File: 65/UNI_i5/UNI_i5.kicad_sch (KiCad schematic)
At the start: 191 parts, among them J2 Conn_01x04, J3 Conn_01x05, SW1 MX_SW_solder, SW10 MX_SW_solder, SW11 MX_SW_solder, SW12 MX_SW_solder, SW13 MX_SW_solder, SW14 MX_SW_solder, SW15 MX_SW_solder, SW16 MX_SW_solder, SW17 MX_SW_solder, SW18 MX_SW_solder, SW19 MX_SW_solder, SW2 MX_SW_solder, SW20 MX_SW_solder, SW21 MX_SW_solder, SW22 MX_SW_solder, SW23 MX_SW_solder, SW24 MX_SW_solder, SW25 MX_SW_solder, SW26 MX_SW_solder, SW27 MX_SW_solder, SW28 MX_SW_solder, SW29 MX_SW_solder, SW3 MX_SW_solder, SW30 MX_SW_solder, SW31 MX_SW_solder, SW32 RotaryEncoder_Switch, SW33 MX_SW_solder, SW34 MX_SW_solder, SW35 MX_SW_solder, SW36 MX_SW_solder, SW37 MX_SW_solder, SW38 MX_SW_solder, SW39 MX_SW_solder, SW4 MX_SW_solder, SW40 MX_SW_solder, SW41 MX_SW_solder, SW42 MX_SW_solder, SW43 MX_SW_solder, SW44 MX_SW_solder, SW45 MX_SW_solder, SW46 MX_SW_solder, SW47 MX_SW_solder, SW48 RotaryEncoder_Switch, SW49 MX_SW_solder, SW5 MX_SW_solder, SW50 MX_SW_solder, SW51 MX_SW_solder, SW52 MX_SW_solder, SW53 MX_SW_solder, SW54 MX_SW_solder, SW55 MX_SW_solder, SW56 MX_SW_solder, SW57 MX_SW_solder, SW58 MX_SW_solder, SW59 MX_SW_solder, SW6 MX_SW_solder, SW60 MX_SW_solder, SW61 MX_SW_solder, SW62 MX_SW_solder, SW63 MX_SW_solder, SW64 MX_SW_solder, SW65 MX_SW_solder, SW66 MX_SW_solder, SW67 MX_SW_solder, SW68 MX_SW_solder, SW69 MX_SW_solder, SW7 MX_SW_solder, SW70 MX_SW_solder, SW71 MX_SW_solder, SW72 MX_SW_solder, SW73 MX_SW_solder, SW74 MX_SW_solder, SW75 MX_SW_solder, SW76 SW_RESET, SW77 SW_BOOTSEL, SW8 MX_SW_solder, SW9 MX_SW_solder, U1 RP2040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

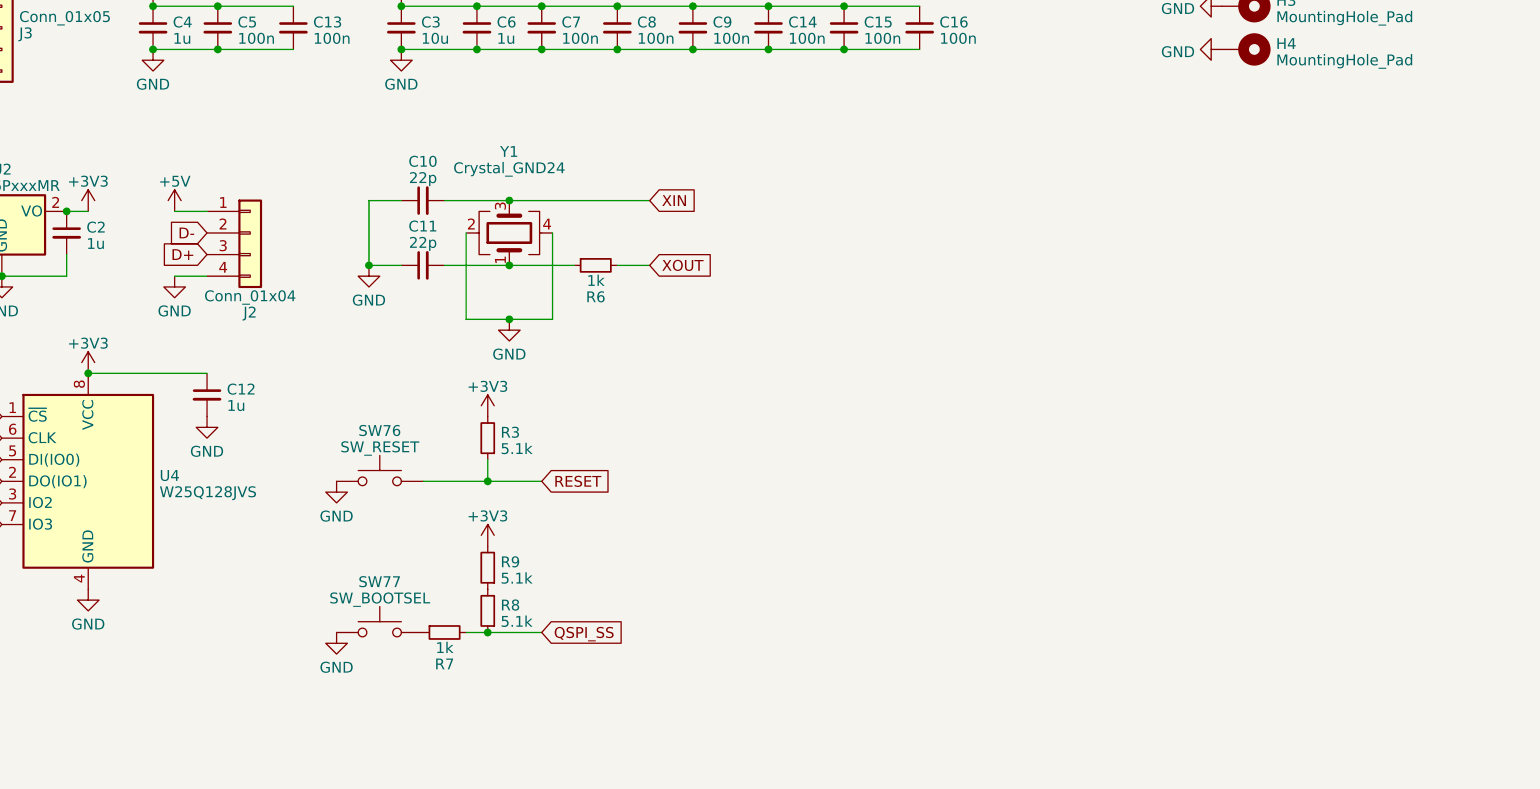
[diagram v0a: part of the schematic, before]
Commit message: 65 v3
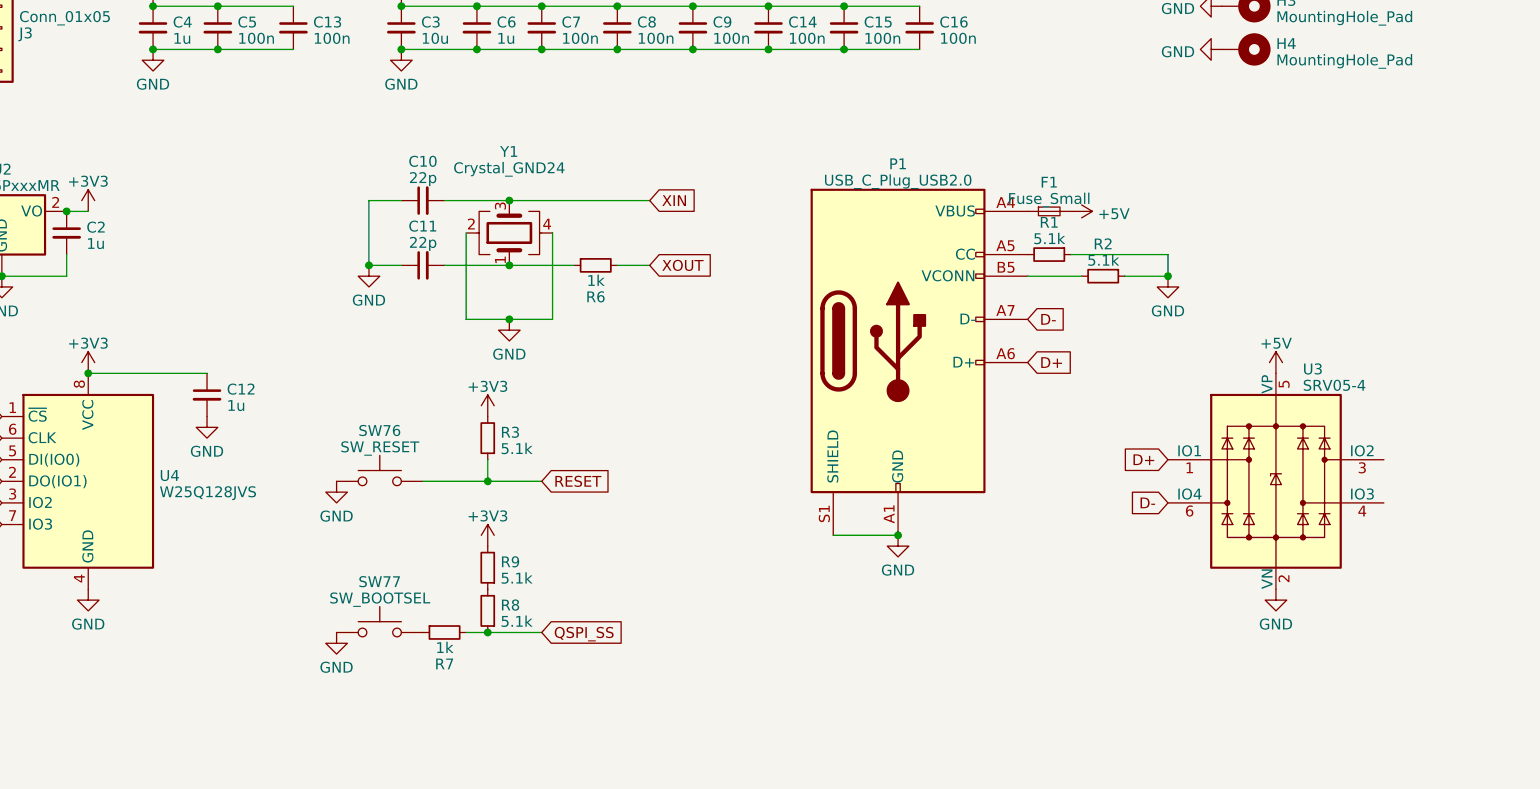
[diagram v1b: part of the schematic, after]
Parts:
- removed J2: Conn_01x04, Connector_Molex:Molex_Pico-EZmate_78171-0004_1x04-1MP_P1.20mm_Vertical, symbol Connector_Generic:Conn_01x04
- added F1: Fuse_Small, Fuse:Fuse_1206_3216Metric, symbol Device:Fuse_Small
- added P1: USB_C_Plug_USB2.0, Connector_USB:USB_C_Receptacle_HRO_TYPE-C-31-M-12, symbol Connector:USB_C_Plug_USB2.0
- added R1, R2: 5.1k, Resistor_SMD:R_0402_1005Metric, symbol Device:R_Small
- added U3: SRV05-4, PCM_marbastlib-various:SOT-23-6-routable, symbol PCM_marbastlib-various:SRV05-4
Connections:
- net +5V: now also F1.2, U3.5 (VP)
- net D+: now also P1.A6 (D+), U3.1 (IO1)
- net D-: now also P1.A7 (D-), U3.6 (IO4)
- net GND: now also P1.A1 (GND), P1.A12 (GND), P1.B1 (GND), P1.B12 (GND), P1.S1 (SHIELD), R1.1, R2.1, U3.2 (VN)
- new net: F1.1, P1.A4 (VBUS), P1.A9 (VBUS), P1.B4 (VBUS), P1.B9 (VBUS)
- new net: P1.B5 (VCONN), R2.2
- new net: P1.A5 (CC), R1.2

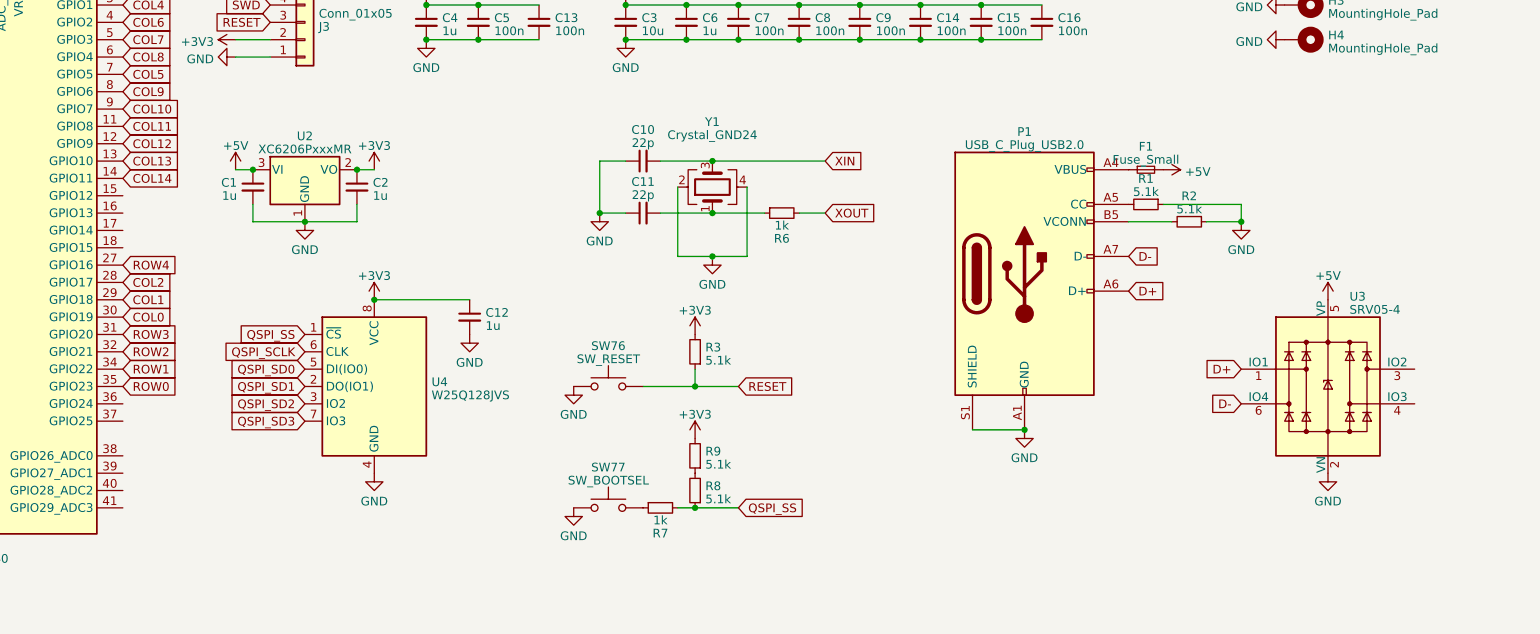
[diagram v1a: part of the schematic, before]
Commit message: v4
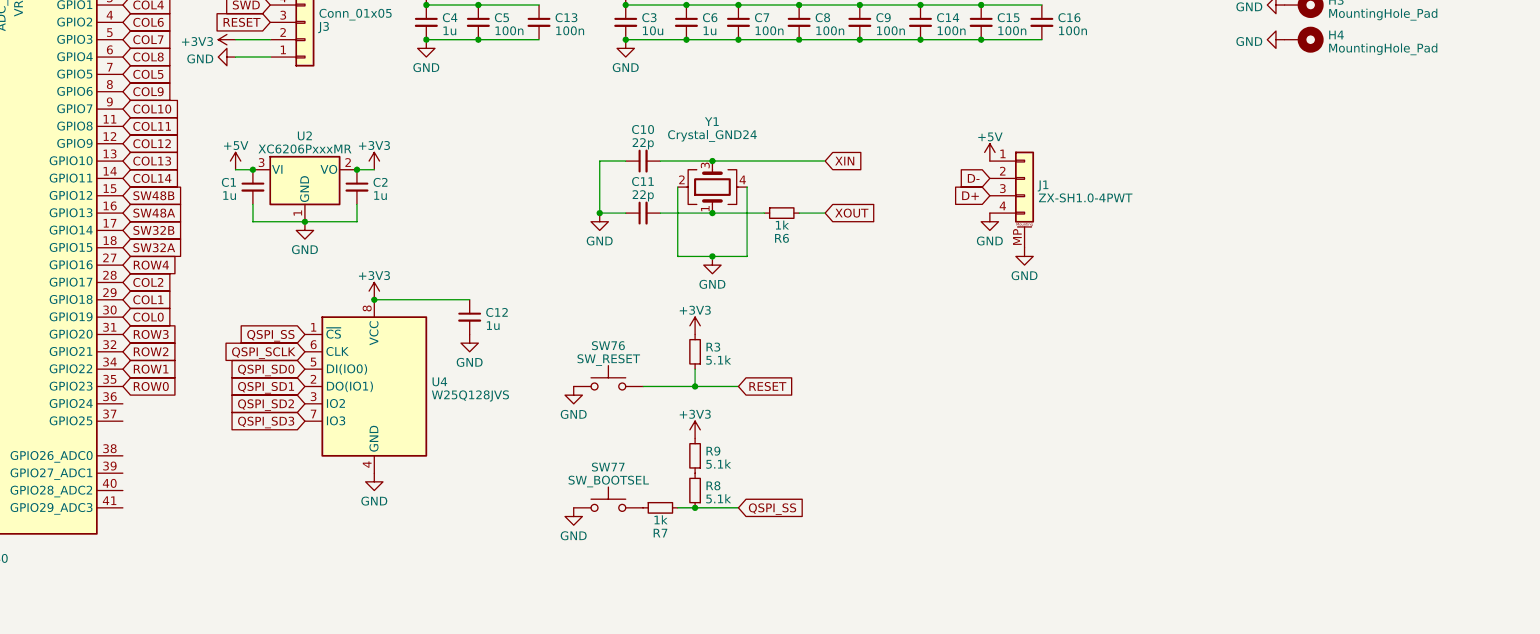
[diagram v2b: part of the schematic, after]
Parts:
- removed F1: Fuse_Small, Fuse:Fuse_1206_3216Metric, symbol Device:Fuse_Small
- removed P1: USB_C_Plug_USB2.0, Connector_USB:USB_C_Receptacle_HRO_TYPE-C-31-M-12, symbol Connector:USB_C_Plug_USB2.0
- removed R1, R2: 5.1k, Resistor_SMD:R_0402_1005Metric, symbol Device:R_Small
- removed U3: SRV05-4, PCM_marbastlib-various:SOT-23-6-routable, symbol PCM_marbastlib-various:SRV05-4
- added J1: ZX-SH1.0-4PWT, Connector_JST:JST_SH_SM04B-SRSS-TB_1x04-1MP_P1.00mm_Horizontal, symbol Connector_Generic_MountingPin:Conn_01x04_MountingPin
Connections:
- net +5V: now also J1.1 (Pin_1)
- net D+: now also J1.3 (Pin_3)
- net D-: now also J1.2 (Pin_2)
- net GND: now also J1.4 (Pin_4), J1.MP (MountPin)
- net SW32A: now also U1.18 (GPIO15)
- net SW32B: now also U1.17 (GPIO14)
- net SW48A: now also U1.16 (GPIO13)
- net SW48B: now also U1.15 (GPIO12)
